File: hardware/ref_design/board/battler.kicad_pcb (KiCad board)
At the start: 2 copper layers, 71.4 x 127.7 mm, 173 parts, among them J1 TYPE-C-31-M-12, J2 53261-0271, J3 FH12-50S-0.5SH(55), J4 53261-0271, J5 SWD, J6 UART, J7 DEBUG PADS, Q1 2N7002, Q2 AO3401A, Q3 2N7002, Q4 2N7002, Q5 AO3400A, Q6 AO3400A, SW1 P1 UP, SW10 P2 DOWN, SW11 P2 LEFT, SW12 P2 RIGHT, SW13 P2 A, SW14 P2 B, SW15 P2 X, SW16 P2 Y, SW18 BOOTSEL, SW19 RESET, SW2 P1 DOWN, SW20 P1 SELECT, SW21 P1 START / PWR, SW22 P2 SELECT, SW23 P2 START, SW3 P1 LEFT, SW4 P1 RIGHT, SW5 P1 A, SW6 P1 B, SW7 P1 X, SW8 P1 Y, SW9 P2 UP, U1 SRV05-4, U2 TP4056-42-ESOP8, U3 ME6211C33M5G, U4 RP2354B, U6 MCP6002, U7 FM8002A, X1 12MHz

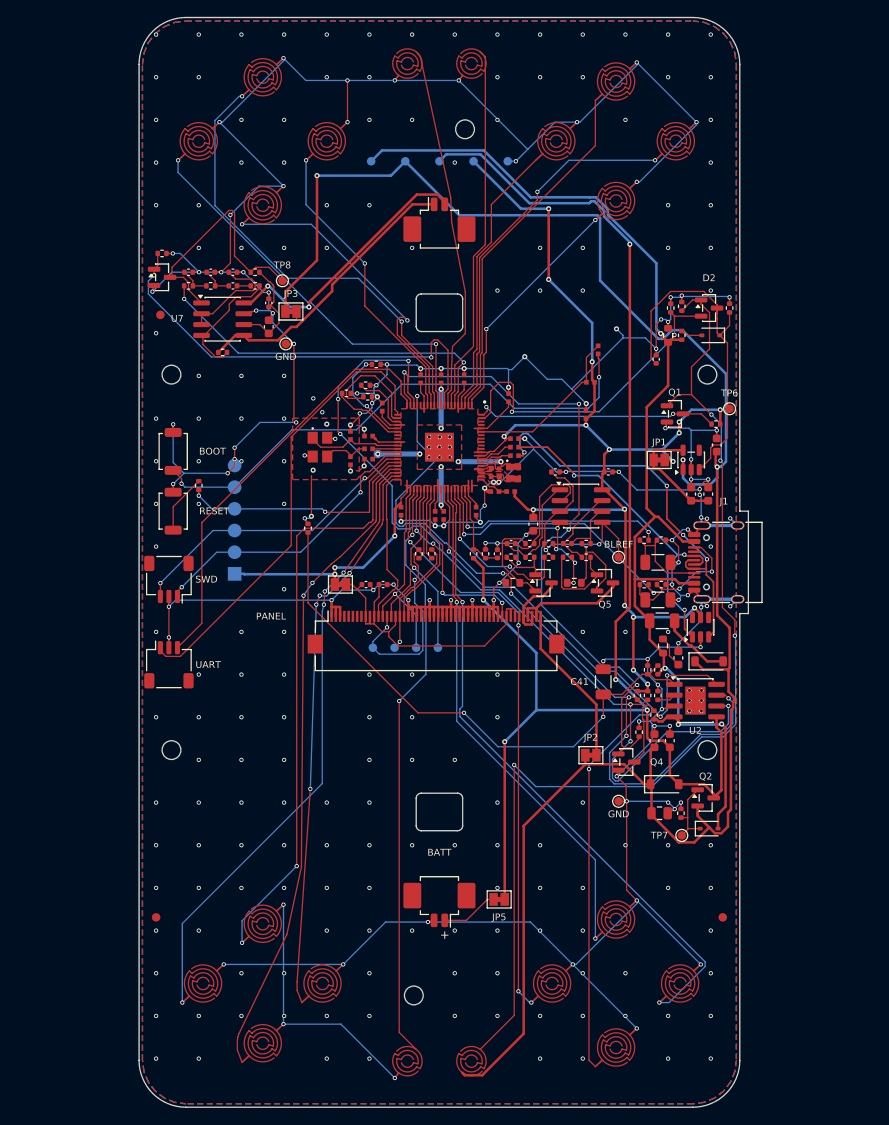
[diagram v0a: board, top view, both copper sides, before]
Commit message: WIP: cell and speaker holes, core on the back (unrouted)
Co-Authored-By: Claude Opus 5.5 <noreply@anthropic.com>
Claude-Session: https://claude.ai/code/session_01Y3mFMxLYqNeyyedvbYuRwX
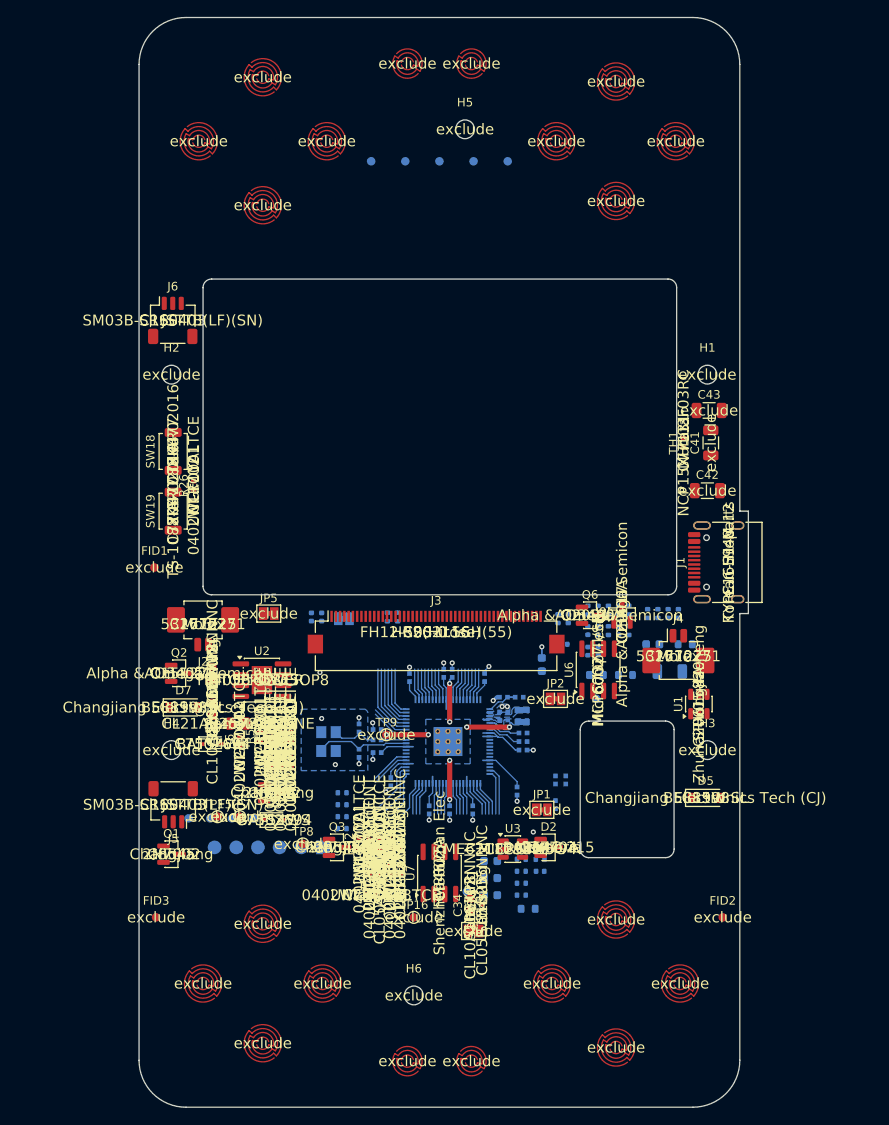
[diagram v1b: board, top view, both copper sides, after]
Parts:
- C1, C10, C11, C12, C13, C14, C15, C16, C17, C18, C19, C20, C21, C22, C23, C24, C25, C26, C27, C28, C29, C30, C47, C48, C49, C5, C50, C51, C6, C7, C8, JP4, L2, R1, R13, R14, R15, R16, R17, R18, R19, R2, R20, R21, R22, R23, R25, R28, R29, R3, R38, R4, R41, R42, R47, R48, R49, R50, R51, R52, R53, R54, R55, R56, R57, R58, R59, R60, R61, TP10, TP6, U4, X1: moved to B.Cu
- TP9: moved to F.Cu
- moved R37 79.1 mm to (92.0, 139.0)
- moved Q1 78.4 mm to (68.6, 134.2)
- moved D3 76.5 mm to (80.6, 130.2), turned to 0 degrees
- moved JP3 75.7 mm to (104.0, 143.2)
- moved C35 74.3 mm to (105.0, 139.6)
- moved C40 72.1 mm to (93.0, 136.0), turned to 90 degrees
- moved C34 71.8 mm to (103.6, 140.2)
- moved R15 71.7 mm to (109.6, 137.6), turned to 180 degrees
- moved R36 71.3 mm to (91.8, 136.0), turned to 90 degrees
- moved R34 70.5 mm to (95.4, 136.0), turned to 90 degrees
- moved C37 70.3 mm to (91.8, 133.0), turned to 90 degrees
- moved C38 70.2 mm to (94.2, 133.0), turned to 90 degrees
- moved Q3 69.9 mm to (88.0, 133.4)
- moved U7 69.7 mm to (100.0, 136.4), turned to 90 degrees
- moved R38 69.2 mm to (110.4, 140.6), turned to 180 degrees
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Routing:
- net GND: track 703.8 -> 12.9 mm, vias 303 -> 22
- net VSYS: track 228.3 -> 0.00 mm, vias 3 -> 0
- net VBAT: track 168.8 -> 0.00 mm, vias 5 -> 0
- net +3V3: track 198.7 -> 37.8 mm, vias 20 -> 0
- net VBUS: track 136.5 -> 0.00 mm, vias 4 -> 0
- net PWR_BTN_RAW: track 125.1 -> 0.00 mm, vias 4 -> 0
- net CHG_DONE_N: track 103.5 -> 3.89 mm, vias 6 -> 0
- net CHG_STAT_N: track 89.9 -> 3.89 mm, vias 6 -> 0
- net P1_B: track 86.1 -> 3.85 mm, vias 2 -> 0
- net CHG_OFF: track 79.1 -> 3.89 mm, vias 4 -> 0
- net P1_A: track 76.8 -> 3.85 mm, vias 2 -> 0
- net P1_DOWN: track 77.2 -> 7.46 mm, vias 2 -> 0
- net P1_LEFT: track 73.6 -> 6.84 mm, vias 4 -> 0
- net P1_Y: track 70.2 -> 3.81 mm, vias 4 -> 0
- net P1_SELECT: track 69.4 -> 3.81 mm, vias 2 -> 0
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- added copper zone on B.Cu, net +1V1
- added copper zone on B.Cu, net +3V3
- added copper zone on B.Cu, net VREG_LX
- removed copper zone on F.Cu, net +1V1
- removed copper zone on F.Cu, net +3V3
- removed copper zone on F.Cu, net GND
- removed copper zone on F.Cu, net VREG_LX
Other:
- outline, holes or cut-outs redrawn
- board text removed: "+"
- board text removed: "1V1"
- board text removed: "2 LAYERS 1.6 MM ENIG"
- board text removed: "3V3"
- board text removed: "BATT"
- board text removed: "BLREF"
- board text removed: "BOOT"
- board text removed: "CELL"
- board text removed: "CS"
- board text removed: "DC"
- board text removed: "GND"
- board text removed: "MOSI"
- board text removed: "PANEL"
- board text removed: "RESET"
- board text removed: "REV 1"
- board text removed: "SCK"
- board text removed: "SPEAKER"
- board text removed: "SPK PLUG"
- board text removed: "SWD"
- board text removed: "SWD PADS"
- board text removed: "TWO-PLAYER HANDHELD REF-A"
- board text removed: "UART"
- board text removed: "VBAT"
- board text removed: "VBUS"
- board text removed: "VSYS"
